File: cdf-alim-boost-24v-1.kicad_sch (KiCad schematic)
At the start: 14 parts, among them J2 Conn_01x02, U1 TPS259470x

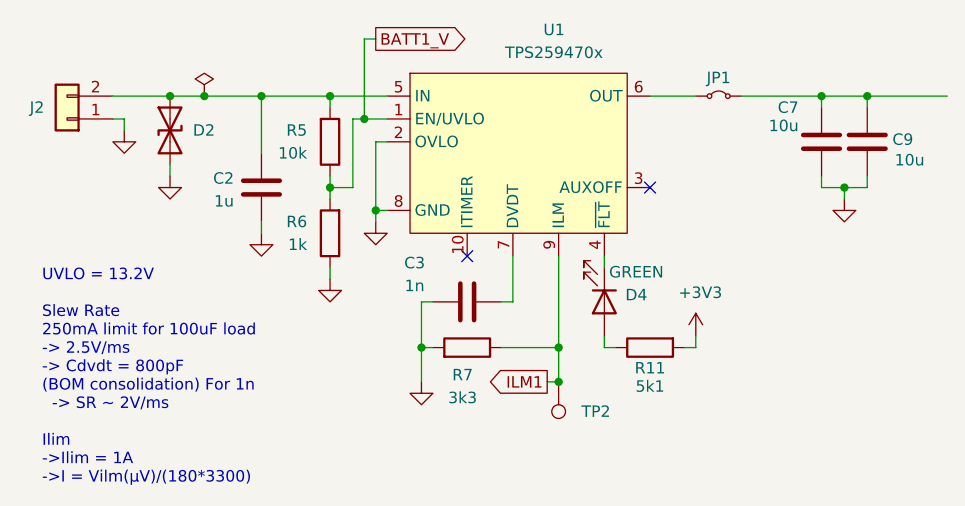
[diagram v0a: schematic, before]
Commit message: schem: remove efuse
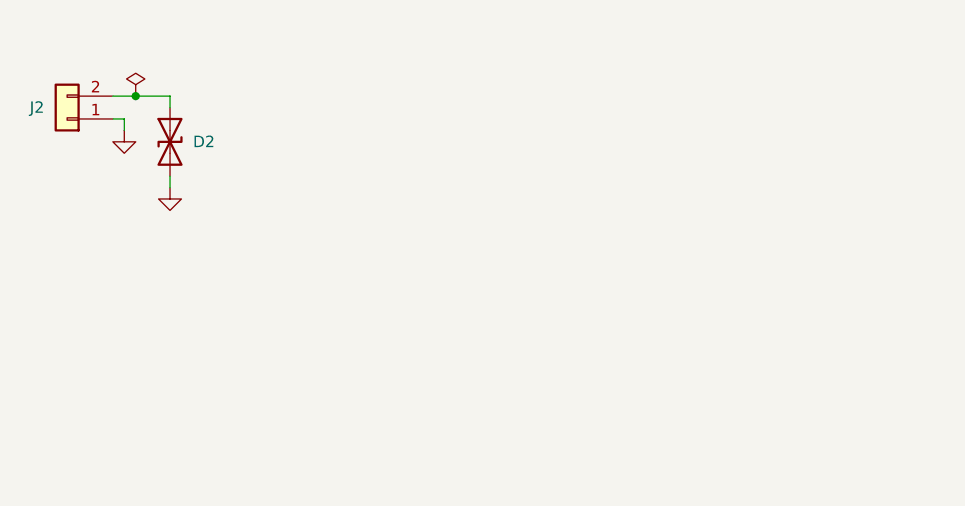
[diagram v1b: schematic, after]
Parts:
- removed C2: 1u, Capacitor_SMD:C_0402_1005Metric, symbol Device:C
- removed C3: 1n, Capacitor_SMD:C_0402_1005Metric, symbol Device:C
- removed C7, C9: 10u, Capacitor_SMD:C_0805_2012Metric, symbol Device:C
- removed D4: GREEN, LED_SMD:LED_0805_2012Metric, symbol Device:LED
- removed JP1: Jumper_2_Small_Bridged, Connector_PinHeader_2.54mm:PinHeader_1x02_P2.54mm_Vertical, symbol Jumper:Jumper_2_Small_Bridged
- removed R11: 5k1, Resistor_SMD:R_0402_1005Metric, symbol Device:R
- removed R5: 10k, Resistor_SMD:R_0402_1005Metric, symbol Device:R
- removed R6: 1k, Resistor_SMD:R_0402_1005Metric, symbol Device:R
- removed R7: 3k3, Resistor_SMD:R_0402_1005Metric, symbol Device:R
- removed TP2: TestPoint, TestPoint:TestPoint_Pad_D2.0mm, symbol Connector:TestPoint
- removed U1: TPS259470x, GLCS:Texas_RPW0010A_VQFN-HR-10_2x2mm_P0.5mm, symbol GLCS:TPS259470x
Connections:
- no-connect marks 2 -> 0
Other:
- note removed: "UVLO = 13.2V Slew Rate 250mA limit for 100uF load -> 2.5V/ms -> Cdvdt = 800pF (BOM consolidation) For 1n -> SR ~ 2V/ms Ilim ->Ilim = 1A ->I = Vilm(µV)/(180*3300)"
- moved on the sheet: D2
